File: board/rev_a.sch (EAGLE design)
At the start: 32 parts, among them IC3 MCP2551, Q1 35A/25V/8.5mΩ

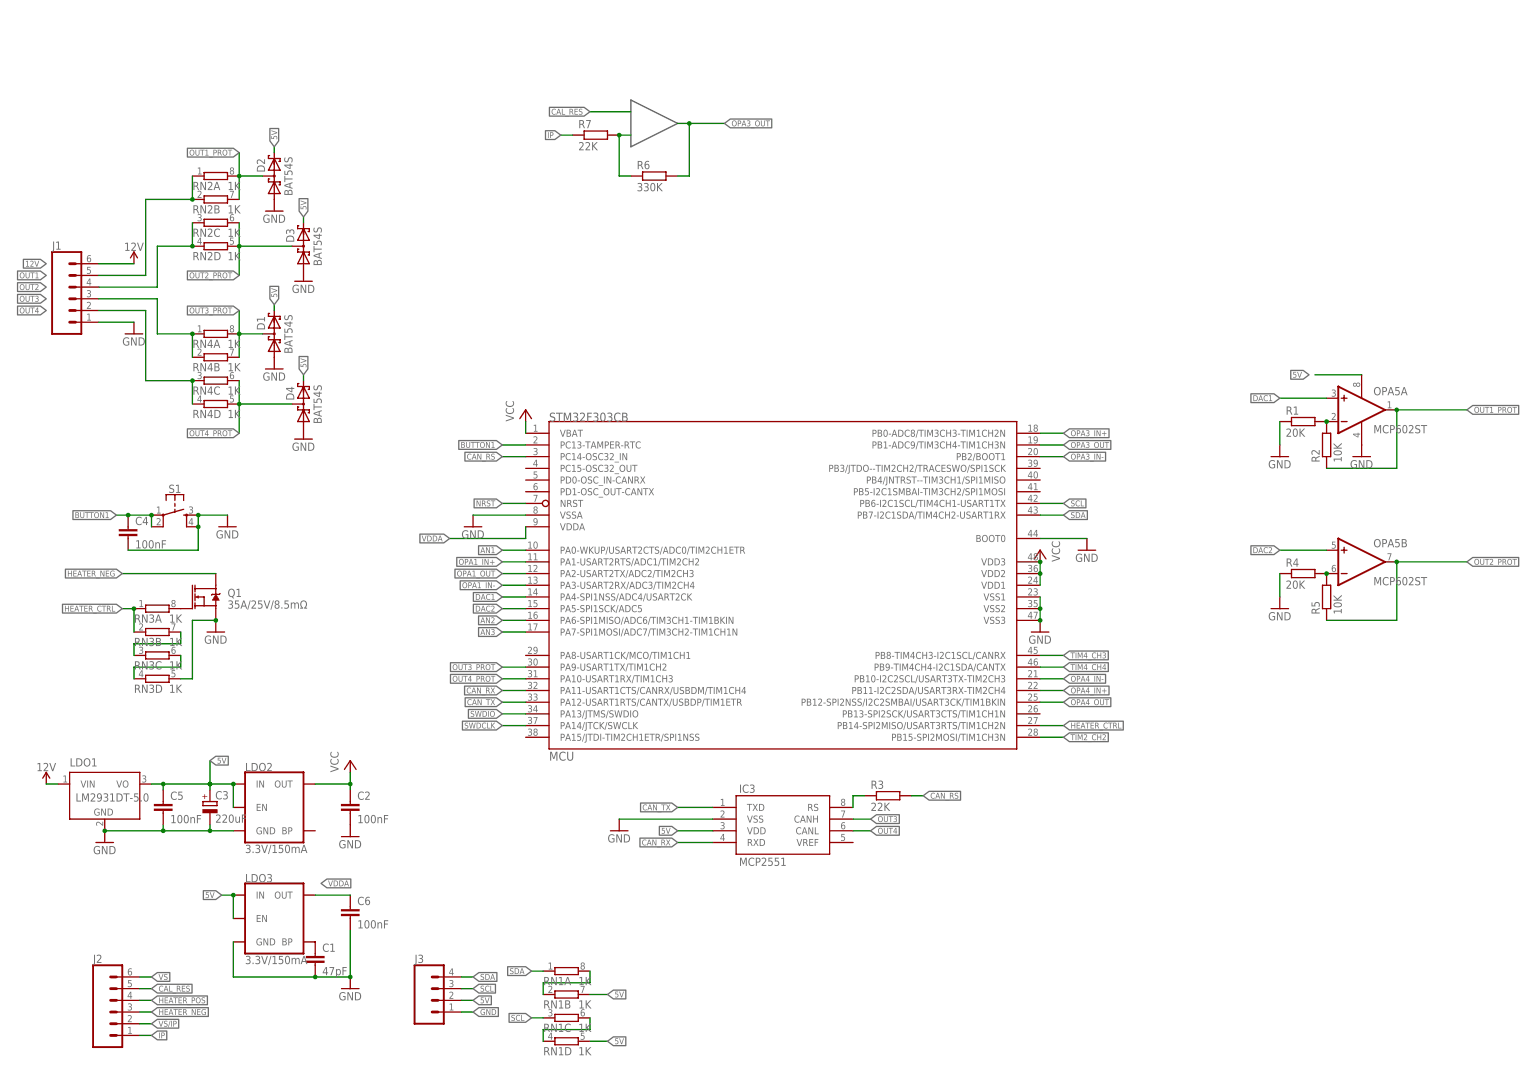
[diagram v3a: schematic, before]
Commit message: [board] Working on schema
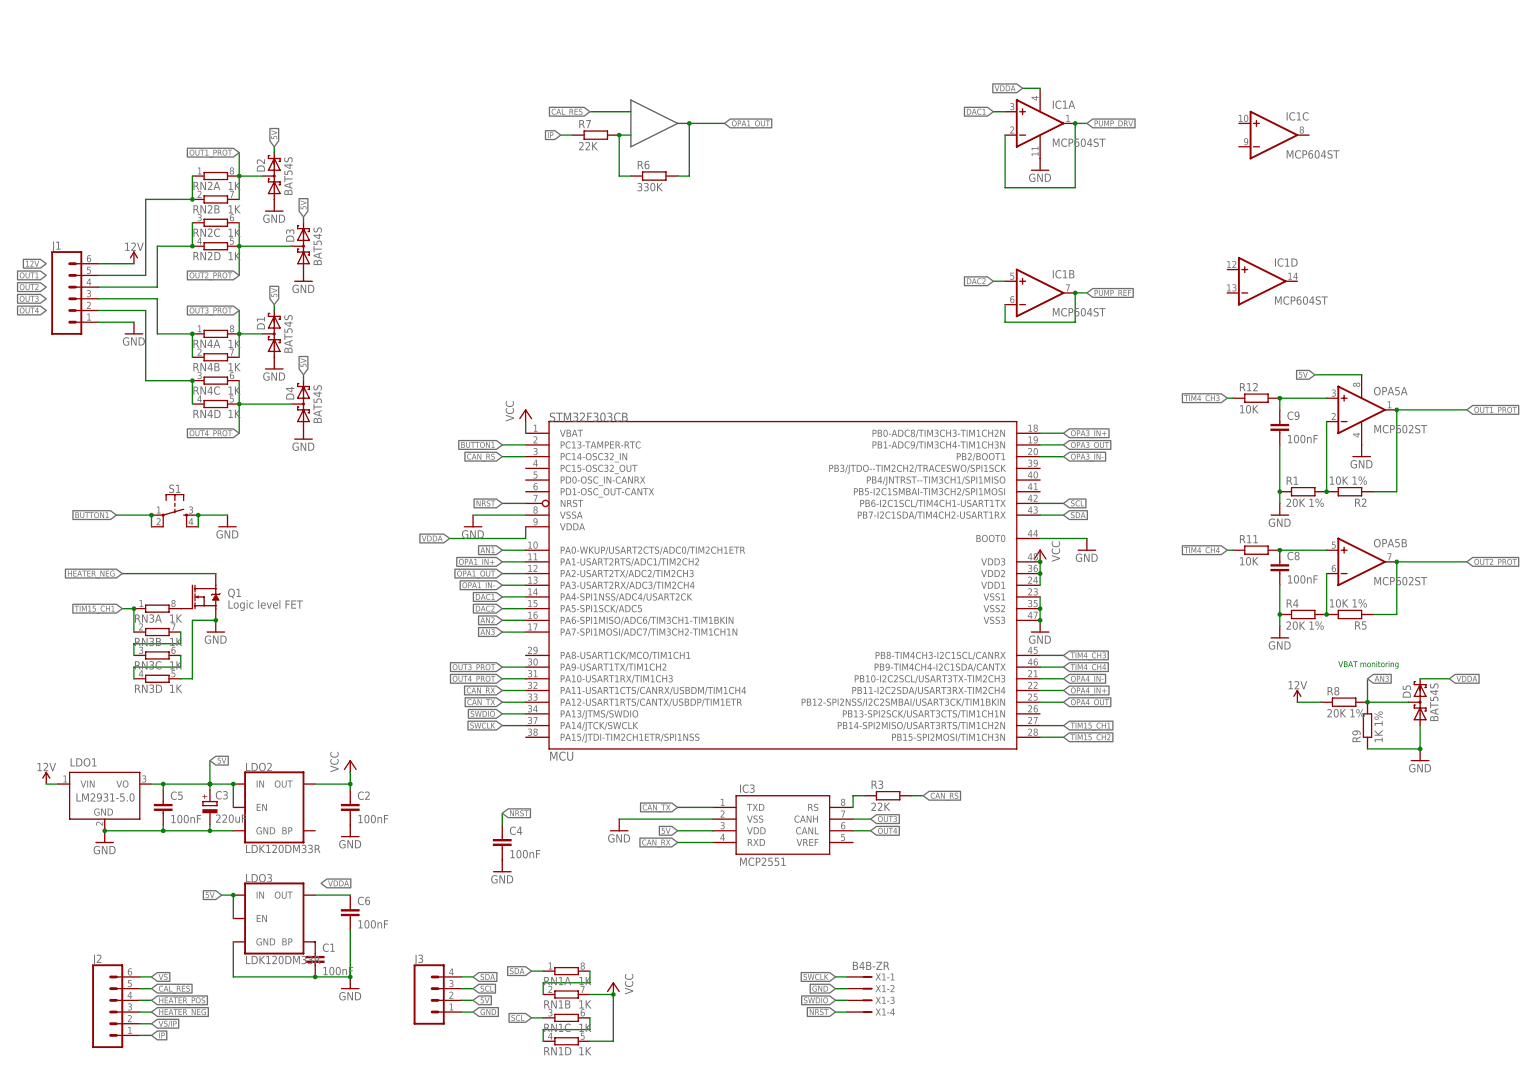
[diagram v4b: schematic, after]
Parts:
- added C8, C9: 100nF, resistor:C-EUC0603
- added D5: BAT54S, diode:BAT54S
- added IC1: MCP604ST, linear:MCP604ST
- added R11, R12: 10K, resistor:R-EU_R0603
- added R8: 20K 1%, resistor:R-EU_R0603
- added R9: 1K 1%, resistor:R-EU_R0603
- added X1: B4B-ZR, con-jst:B4B-ZR
- C1: value 47pF -> 100nF
- LDO1: value LM2931DT-5.0 -> LM2931-5.0
- LDO2, LDO3: value 3.3V/150mA -> LDK120DM33R
- Q1: value 35A/25V/8.5mΩ -> Logic level FET
- R1, R4: value 20K -> 20K 1%
- R2, R5: value 10K -> 10K 1%
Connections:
- net HEATER_CTRL renamed TIM15_CH1
- net TIM2_CH2 renamed TIM15_CH2
- removed net SWDCLK: MCU.PA14/JTCK/SWCLK
- new net N$13: C9.1, OPA5A.+IN, R12.2
- new net N$4: C8.1, OPA5B.+IN, R11.2
- new net PUMP_DRV: IC1A.-IN, IC1A.OUT
- new net PUMP_REF: IC1B.-IN, IC1B.OUT
- new net SWCLK: MCU.PA14/JTCK/SWCLK, X1-1.1
- net 12V: now also R8.1
- net 5V: no longer RN1B.2, RN1D.2
- net AN3: now also D5.C1A2, R8.2, R9.2
- net BUTTON1: no longer C4.1
- net DAC1: now also IC1A.+IN; no longer OPA5A.+IN
- net DAC2: now also IC1B.+IN; no longer OPA5B.+IN
- net GND: now also C8.2, C9.2, D5.A1, IC1P.V-, R9.1, X1-2.1
- net N$6: now also OPA5B.-IN
- net NRST: now also C4.1, X1-4.1
- net OPA1_OUT: now also R6.2
- net OPA3_OUT: no longer R6.2
- net SWDIO: now also X1-3.1
- net TIM4_CH3: now also R12.1
- net TIM4_CH4: now also R11.1
- net VCC: now also RN1B.2, RN1D.2
- net VDDA: now also D5.C2, IC1P.V+
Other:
- note added: "OPA1"
- note added: "VBAT monitoring"
- note removed: "OPA3"
- moved on the sheet: C4, R1, R2, R4, R5
